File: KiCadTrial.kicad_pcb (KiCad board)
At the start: 2 copper layers, 13 x 16 mm, 3 parts, among them J1 Conn_01x02

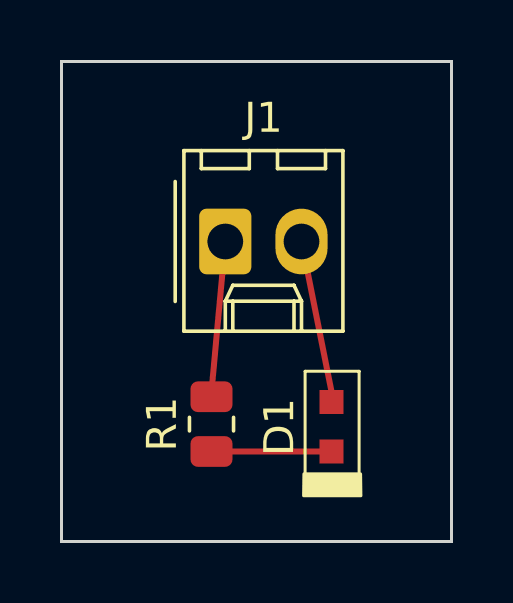
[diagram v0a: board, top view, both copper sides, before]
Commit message: Changes by Lee.
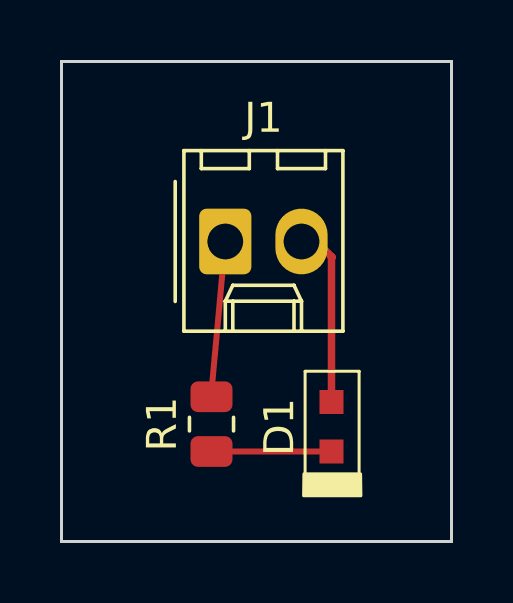
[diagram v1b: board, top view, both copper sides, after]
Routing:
- net GND: track 0.00 -> 6.07 mm
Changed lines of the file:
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@@
     )
   )
-  (gr_line (start 160 109) (end 159 104)
-    (stroke (width 0.2) (type default)) (layer "F.Cu"))
   (gr_line (start 156 109) (end 156.46 104)
     (stroke (width 0.2) (type default)) (layer "F.Cu"))
@@
   (gr_line (start 151 98) (end 164 98)
     (stroke (width 0.1) (type default)) (layer "Edge.Cuts"))
+  (segment (start 160.02 104.521) (end 160 104.541) (width 0.25) (layer "F.Cu") (net 1))
+  (segment (start 159.499 104) (end 160.02 104.521) (width 0.25) (layer "F.Cu") (net 1))
+  (segment (start 160 104.541) (end 160 109.35) (width 0.25) (layer "F.Cu") (net 1))
+  (segment (start 159 104) (end 159.499 104) (width 0.25) (layer "F.Cu") (net 1))
 )
